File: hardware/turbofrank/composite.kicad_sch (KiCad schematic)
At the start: 16 parts, among them J19 RCA-103

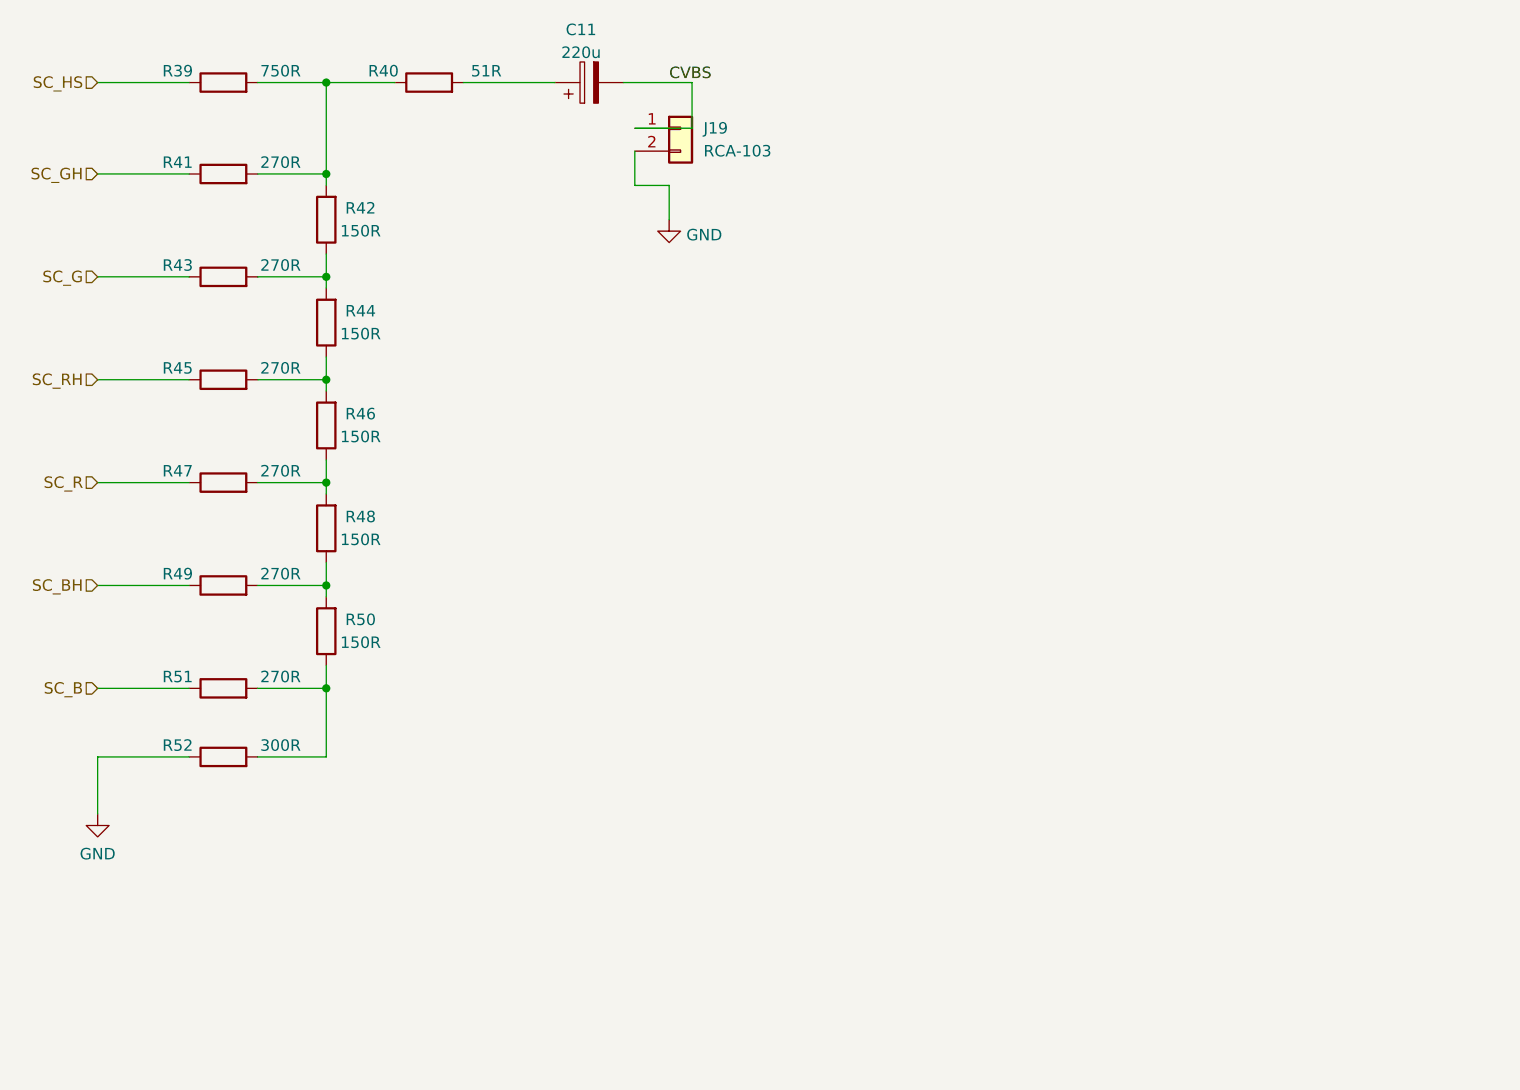
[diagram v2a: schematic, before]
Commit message: TurboFRANK HW 1.05 Release
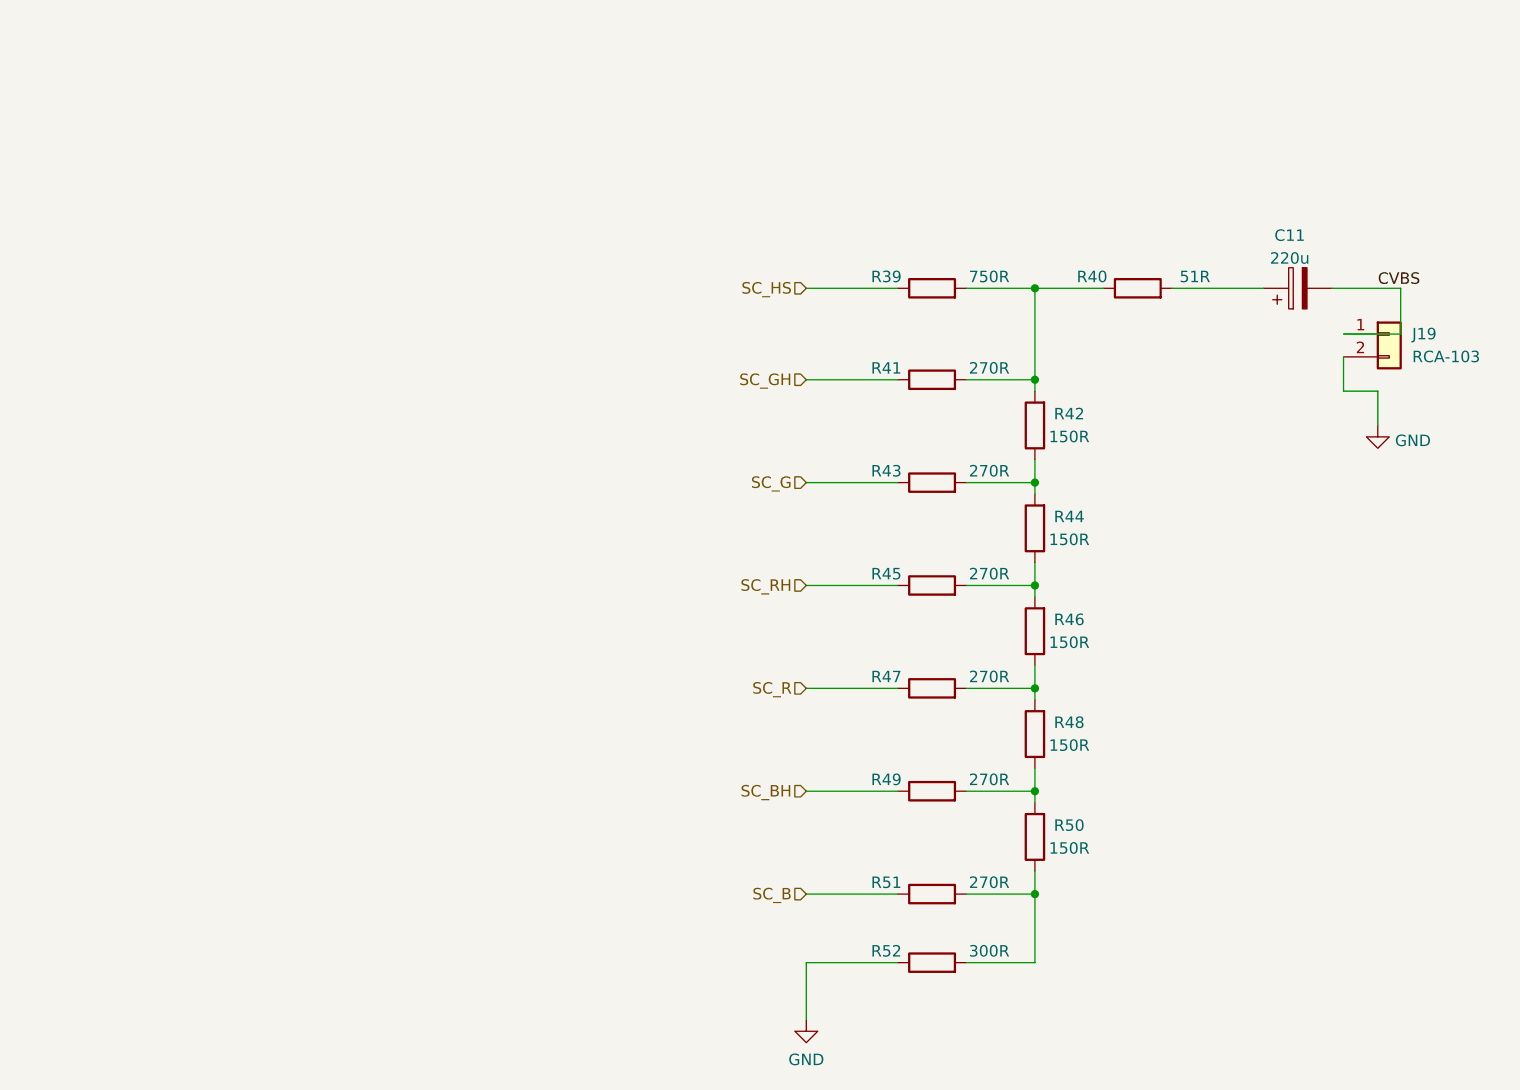
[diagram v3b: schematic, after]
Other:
- moved on the sheet: C11, J19, R39, R40, R41, R42, R43, R44, R45, R46, R47, R48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

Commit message: Bugfixes
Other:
- title: TurboFRANK -> ${NAME}
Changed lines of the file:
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@@
 	(paper "A4")
 	(title_block
-		(title "TurboFRANK")
-		(date "2025-04-04")
+		(title "${NAME}")
+		(date "2025-04-20")
 		(rev "${VERSION}")
 		(company "Mikhail Matveev")
